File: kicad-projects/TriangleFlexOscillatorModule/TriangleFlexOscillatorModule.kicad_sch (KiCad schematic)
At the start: 8 parts

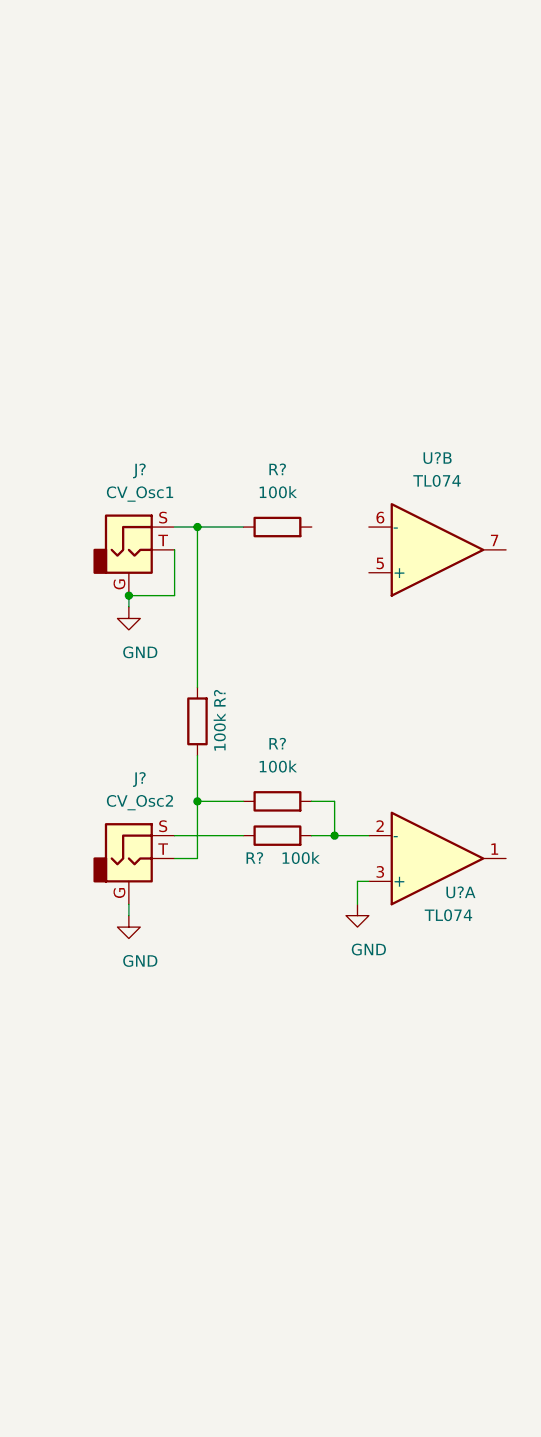
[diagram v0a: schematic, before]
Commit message: Committed some uncommitted changes
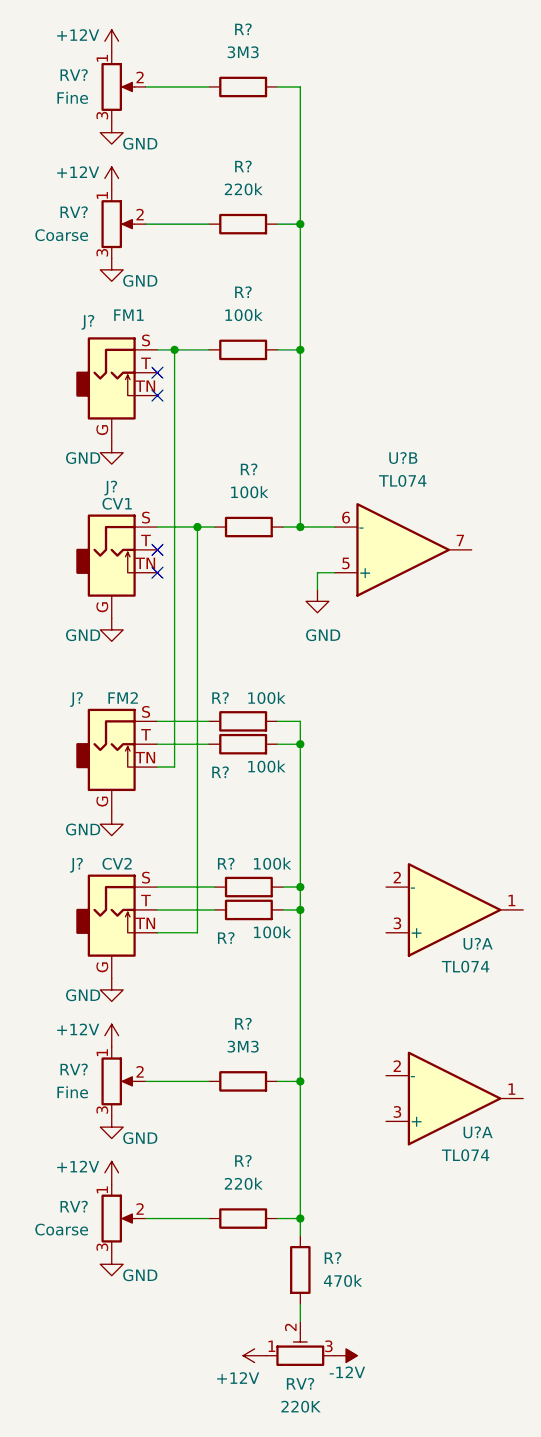
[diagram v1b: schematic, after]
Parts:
- removed J?: CV_Osc1, symbol Connector:AudioJack2_Ground
- removed J?: CV_Osc2, symbol Connector:AudioJack2_Ground
- removed R? (x4): 100k, symbol Device:R
- added J?: FM2, symbol Connector:AudioJack2_Ground_SwitchT
- added J?: FM1, symbol Connector:AudioJack2_Ground_SwitchT
- added J?: CV2, symbol Connector:AudioJack2_Ground_SwitchT
- added J?: CV1, symbol Connector:AudioJack2_Ground_SwitchT
- added R? (x2): 220k, symbol Device:R
- added R? (x6): 100k, symbol Device:R
- added R? (x2): 3M3, symbol Device:R
- added R?: 470k, symbol Device:R
- added RV? (x2): Coarse, symbol Device:R_Potentiometer
- added RV? (x2): Fine, symbol Device:R_Potentiometer
- added RV?: 220K, symbol Device:R_Potentiometer_Trim
- added U?: TL074, symbol Amplifier_Operational:TL074
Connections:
- net GND: now also U?.5 (+), J?.G, J?.G, J?.G, J?.G, RV?.3, RV?.3, RV?.3, RV?.3; no longer U?.3 (+)
- net at U?.6 (-): now also R?.2, R?.2, R?.2, R?.2
- new net: J?.S, R?.1 (x2)
- new net: J?.T, R?.1 (x2)
- new net: J?.S, J?.TN, R?.1 (x2)
- new net: R?.1, RV?.2 (x4)
- new net: R?.1, R?.2, R?.2, R?.2, R?.2, R?.2, R?.2
- new net: R?.2, RV?.2
- new net +12V: RV?.1, RV?.1, RV?.1, RV?.1, RV?.1
- new net -12V: RV?.3
- no-connect marks 0 -> 4
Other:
- moved on the sheet: U?A, U?B
